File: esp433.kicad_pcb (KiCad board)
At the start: 2 copper layers, 47.1 x 72.6 mm, 47 parts, among them J1 USB_OTG, J2 CONN_01X03, Q1 MBT2222ADW1T1, SW1 SW_Push, U1 IRM-02-5, U2 AP2127K-3.3, U3 MAX7044, U4 ESP-12E, U5 FT231XS, Y1 Crystal

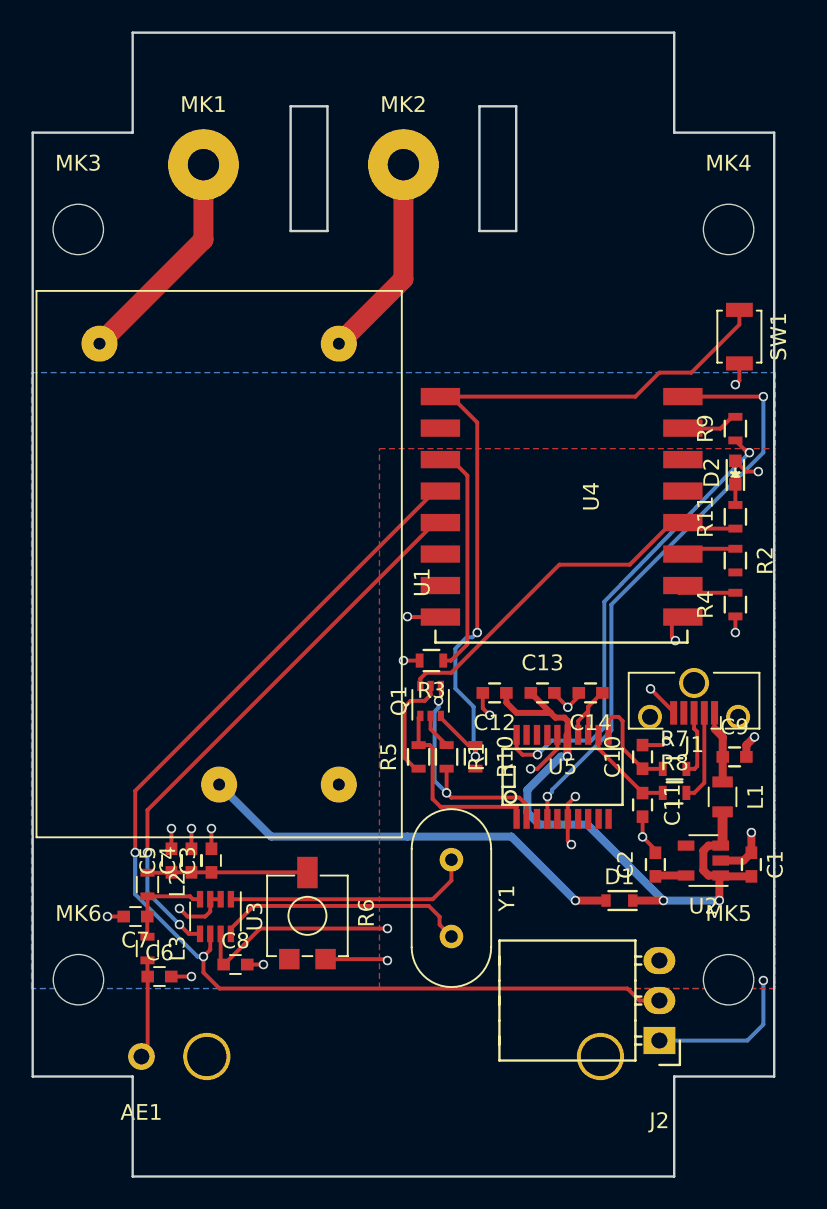
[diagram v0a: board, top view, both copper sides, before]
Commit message: Rearrange silk
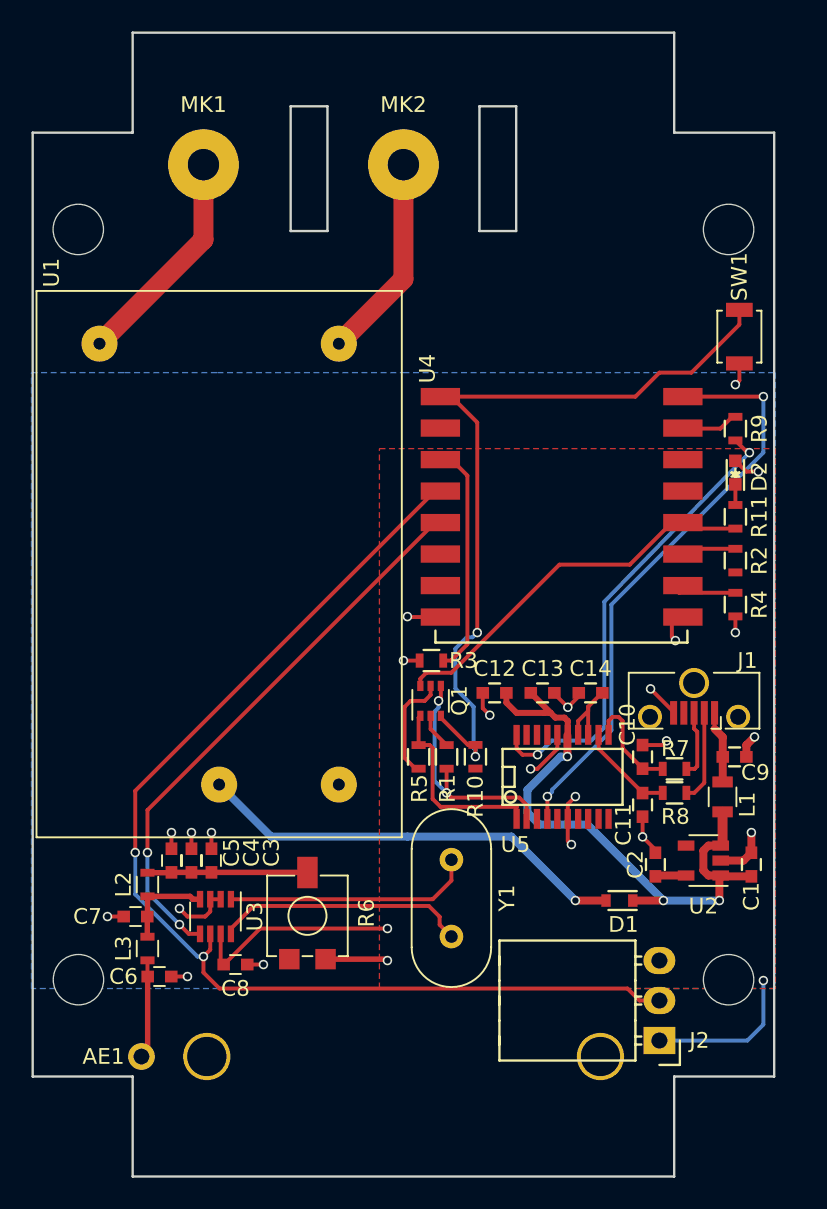
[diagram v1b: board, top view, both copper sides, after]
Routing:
- net GND: track 47.1 -> 46.1 mm
